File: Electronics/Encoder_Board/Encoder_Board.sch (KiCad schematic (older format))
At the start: 4 parts, among them K1 CONN_3

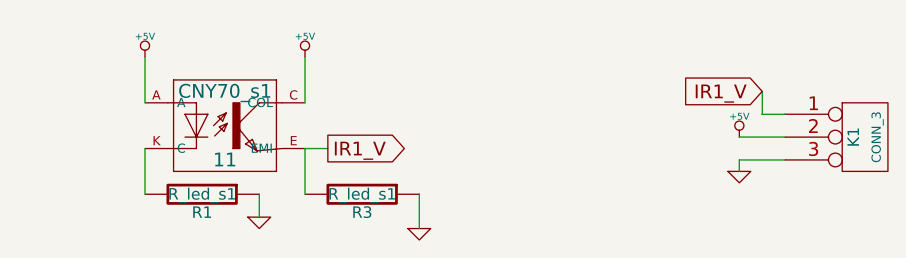
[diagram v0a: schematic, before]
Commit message: Finished encoder board
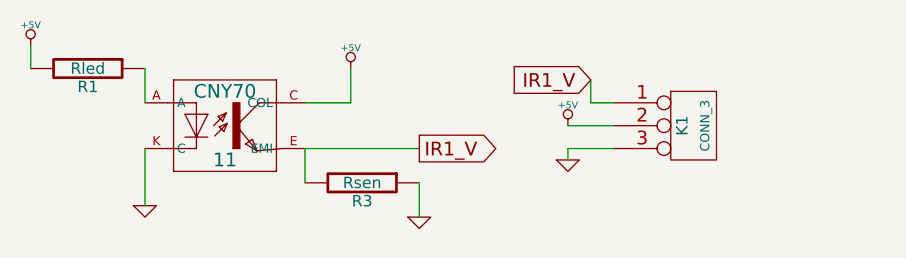
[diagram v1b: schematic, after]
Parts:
- 11: value CNY70_s1 -> CNY70
- R1: value R_led_s1 -> Rled
- R3: value R_led_s1 -> Rsen
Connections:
- net +5V: now also R1.2; no longer 11.A
- net GND: now also 11.K (C); no longer R1.1
- new net: 11.A, R1.1
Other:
- moved on the sheet: K1, R1, R3
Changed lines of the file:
@@
-EESchema Schematic File Version 2  date Mon 17 Jun 2013 16:27:06 CEST
-LIBS:/home/carlosgs/GitRepos/GNBot/Electronics/KicadLibs/CNY0_HERDproject/cny70,power,device,transistors,conn,linear,regul,74xx,cmos4000,adc-dac,memory,xilinx,special,microcontrollers,dsp,microchip,analog_switches,motorola,texas,intel,audio,interface,digital-audio,philips,display,cypress,siliconi,opto,atmel,contrib,valves,./Encoder_Board.cache
-EELAYER 24  0
+EESchema Schematic File Version 2  date lun 17 jun 2013 19:47:10 CEST
+LIBS:cny70
+LIBS:power
+LIBS:device
+LIBS:transistors
+LIBS:conn
+LIBS:linear
+LIBS:regul
+LIBS:74xx
+LIBS:cmos4000
+LIBS:adc-dac
+LIBS:memory
+LIBS:xilinx
+LIBS:special
+LIBS:microcontrollers
+LIBS:dsp
+LIBS:microchip
+LIBS:analog_switches
+LIBS:motorola
+LIBS:texas
+LIBS:intel
+LIBS:audio
+LIBS:interface
+LIBS:digital-audio
+LIBS:philips
+LIBS:display
+LIBS:cypress
+LIBS:siliconi
+LIBS:opto
+LIBS:atmel
+LIBS:contrib
+LIBS:valves
+LIBS:Encoder_Board-cache
+EELAYER 24 0
 EELAYER END
-$Descr A4 11700 8267
+$Descr A4 11693 8268
+encoding utf-8
 Sheet 1 1
 Title ""
@@
 $EndDescr
 Wire Wire Line
-	4550 1900 4550 1850
+	3800 1850 3800 1800
 Wire Wire Line
-	4550 1850 4750 1850
+	3800 1800 4000 1800
 Wire Wire Line
-	4650 1550 4650 1650
+	3900 1500 3900 1600
 Wire Wire Line
-	4650 1650 4750 1650
+	3900 1600 4000 1600
 Wire Wire Line
-	2750 1800 2650 1800
-Wire Wire Line
-	2650 1800 2650 2000
-Wire Wire Line
-	2450 2000 2450 2100
-Wire Wire Line
-	2650 1400 2650 1600
-Wire Wire Line
-	1950 1400 1950 1600
-Wire Wire Line
-	3150 2000 3150 2150
-Wire Wire Line
-	1950 1800 1950 2000
-Wire Wire Line
-	4750 1750 4550 1750
+	4000 1700 3800 1700
 $Comp
 L CONN_3 K1
 U 1 1 51BF17EB
-P 5100 1750
-F 0 "K1" V 5050 1750 50  0000 C CNN
-F 1 "CONN_3" V 5150 1750 40  0000 C CNN
-	1    5100 1750
+P 4350 1700
+F 0 "K1" V 4300 1700 50  0000 C CNN
+F 1 "CONN_3" V 4400 1700 40  0000 C CNN
+F 2 "" H 4350 1700 60  0001 C CNN
+F 3 "" H 4350 1700 60  0001 C CNN
+	1    4350 1700
 	1    0    0    -1
 $EndComp
-Text GLabel 2750 1800 2    60   Output ~ 0
+Text GLabel 3150 1800 2    60   Output ~ 0
 IR1_V
 $Comp
 L GND #PWR01
 U 1 1 51BF1253
-P 3150 2150
-F 0 "#PWR01" H 3150 2150 30  0001 C CNN
-F 1 "GND" H 3150 2080 30  0001 C CNN
-	1    3150 2150
+P 3150 2100
+F 0 "#PWR01" H 3150 2100 30  0001 C CNN
+F 1 "GND" H 3150 2030 30  0001 C CNN
+F 2 "" H 3150 2100 60  0001 C CNN
+F 3 "" H 3150 2100 60  0001 C CNN
+	1    3150 2100
 	1    0    0    -1
 $EndComp
@@
 L GND #PWR02
 U 1 1 51BF1252
-P 2450 2100
-F 0 "#PWR02" H 2450 2100 30  0001 C CNN
-F 1 "GND" H 2450 2030 30  0001 C CNN
-	1    2450 2100
+P 1950 2050
+F 0 "#PWR02" H 1950 2050 30  0001 C CNN
+F 1 "GND" H 1950 1980 30  0001 C CNN
+F 2 "" H 1950 2050 60  0001 C CNN
+F 3 "" H 1950 2050 60  0001 C CNN
+	1    1950 2050
 	1    0    0    -1
 $EndComp
@@
 L +5V #PWR03
 U 1 1 51BF1251
-P 2650 1400
-F 0 "#PWR03" H 2650 1490 20  0001 C CNN
-F 1 "+5V" H 2650 1490 30  0000 C CNN
-	1    2650 1400
+P 2850 1450
+F 0 "#PWR03" H 2850 1540 20  0001 C CNN
+F 1 "+5V" H 2850 1540 30  0000 C CNN
+F 2 "" H 2850 1450 60  0001 C CNN
+F 3 "" H 2850 1450 60  0001 C CNN
+	1    2850 1450
 	1    0    0    -1
 $EndComp
@@
 L +5V #PWR04
 U 1 1 51BF1250
-P 1950 1400
-F 0 "#PWR04" H 1950 1490 20  0001 C CNN
-F 1 "+5V" H 1950 1490 30  0000 C CNN
-	1    1950 1400
+P 1450 1350
+F 0 "#PWR04" H 1450 1440 20  0001 C CNN
+F 1 "+5V" H 1450 1440 30  0000 C CNN
+F 2 "" H 1450 1350 60  0001 C CNN
+F 3 "" H 1450 1350 60  0001 C CNN
+	1    1450 1350
 	1    0    0    -1
 $EndComp
@@
 L R R1
 U 1 1 51BF124F
-P 2200 2000
-F 0 "R1" V 2280 2000 50  0000 C CNN
-F 1 "R_led_s1" V 2200 2000 50  0000 C CNN
-	1    2200 2000
+P 1700 1450
+F 0 "R1" V 1780 1450 50  0000 C CNN
+F 1 "Rled" V 1700 1450 50  0000 C CNN
+F 2 "" H 1700 1450 60  0001 C CNN
+F 3 "" H 1700 1450 60  0001 C CNN
+	1    1700 1450
 	0    1    1    0
 $EndComp
@@
 L R R3
 U 1 1 51BF124E
-P 2900 2000
-F 0 "R3" V 2980 2000 50  0000 C CNN
-F 1 "R_led_s1" V 2900 2000 50  0000 C CNN
-	1    2900 2000
+P 2900 1950
+F 0 "R3" V 2980 1950 50  0000 C CNN
+F 1 "Rsen" V 2900 1950 50  0000 C CNN
+F 2 "" H 2900 1950 60  0001 C CNN
+F 3 "" H 2900 1950 60  0001 C CNN
+	1    2900 1950
 	0    1    1    0
 $EndComp
@@
 AR Path="/51BF124D" Ref="11"  Part="1"
 F 0 "11" H 2300 1550 60  0000 C CNN
-F 1 "CNY70_s1" H 2300 1850 60  0000 C CNN
+F 1 "CNY70" H 2300 1850 60  0000 C CNN
+F 2 "" H 2350 1700 60  0001 C CNN
+F 3 "" H 2350 1700 60  0001 C CNN
 	1    2350 1700
 	1    0    0    -1
@@
 L GND #PWR05
 U 1 1 51BF1143
-P 4550 1900
-F 0 "#PWR05" H 4550 1900 30  0001 C CNN
-F 1 "GND" H 4550 1830 30  0001 C CNN
-	1    4550 1900
+P 3800 1850
+F 0 "#PWR05" H 3800 1850 30  0001 C CNN
+F 1 "GND" H 3800 1780 30  0001 C CNN
+F 2 "" H 3800 1850 60  0001 C CNN
+F 3 "" H 3800 1850 60  0001 C CNN
+	1    3800 1850
 	1    0    0    -1
 $EndComp
@@
 L +5V #PWR06
 U 1 1 51BF113E
-P 4550 1750
-F 0 "#PWR06" H 4550 1840 20  0001 C CNN
-F 1 "+5V" H 4550 1840 30  0000 C CNN
-	1    4550 1750
+P 3800 1700
+F 0 "#PWR06" H 3800 1790 20  0001 C CNN
+F 1 "+5V" H 3800 1790 30  0000 C CNN
+F 2 "" H 3800 1700 60  0001 C CNN
+F 3 "" H 3800 1700 60  0001 C CNN
+	1    3800 1700
 	1    0    0    -1
 $EndComp
-Text GLabel 4650 1550 0    60   Input ~ 0
+Text GLabel 3900 1500 0    60   Input ~ 0
 IR1_V
+Wire Wire Line
+	2650 1800 2650 1950
+Wire Wire Line
+	3150 1950 3150 2100
+Wire Wire Line
+	3150 1800 2650 1800
+Wire Wire Line
+	2850 1450 2850 1600
+Wire Wire Line
+	2850 1600 2650 1600
+Wire Wire Line
+	1950 2050 1950 1800
+Wire Wire Line
+	1950 1600 1950 1450
+Wire Wire Line
+	1450 1450 1450 1350
 $EndSCHEMATC
